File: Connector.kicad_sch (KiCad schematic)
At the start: 13 parts, among them J10 JST_XH_S2B-A, J3 JST_XH_S4B-A, J4 JST_XH_S2B-A, J5 JST_XH_S2B-A, J6 JST_XH_S2B-A, J7 JST_XH_S2B-A, J8 JST_XH_S3B, SW2 OS102011MA1Q, U13 74LVC2G126

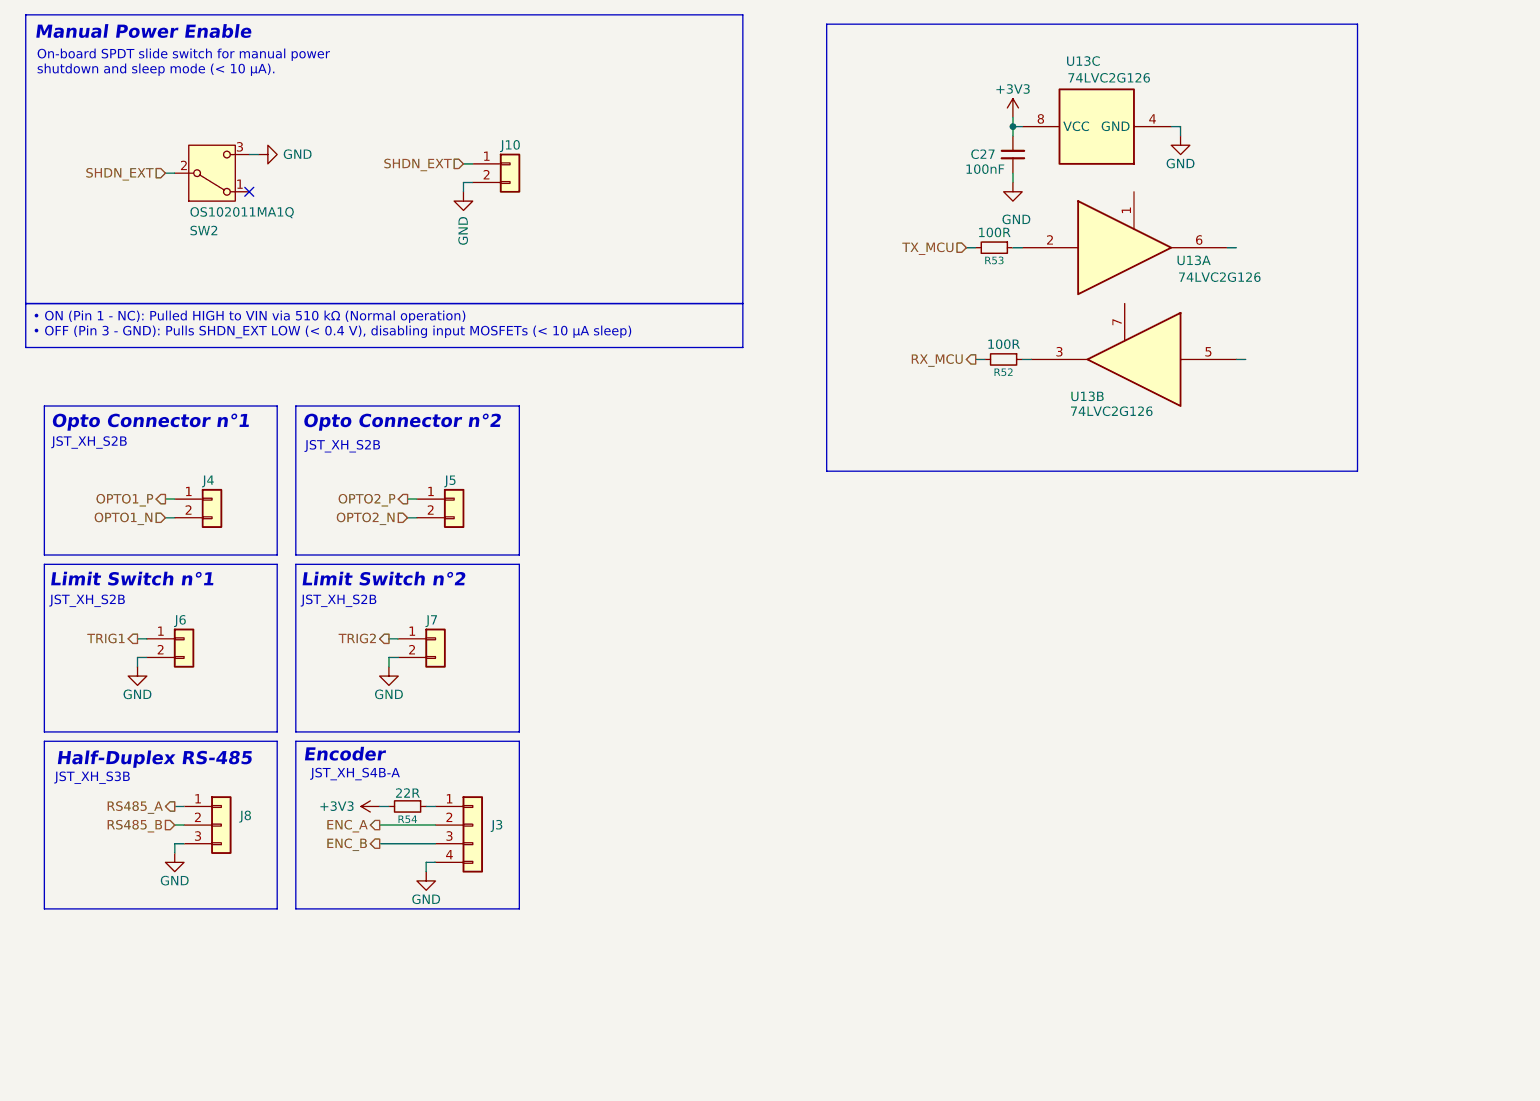
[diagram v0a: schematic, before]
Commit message: fix: FIx some modification
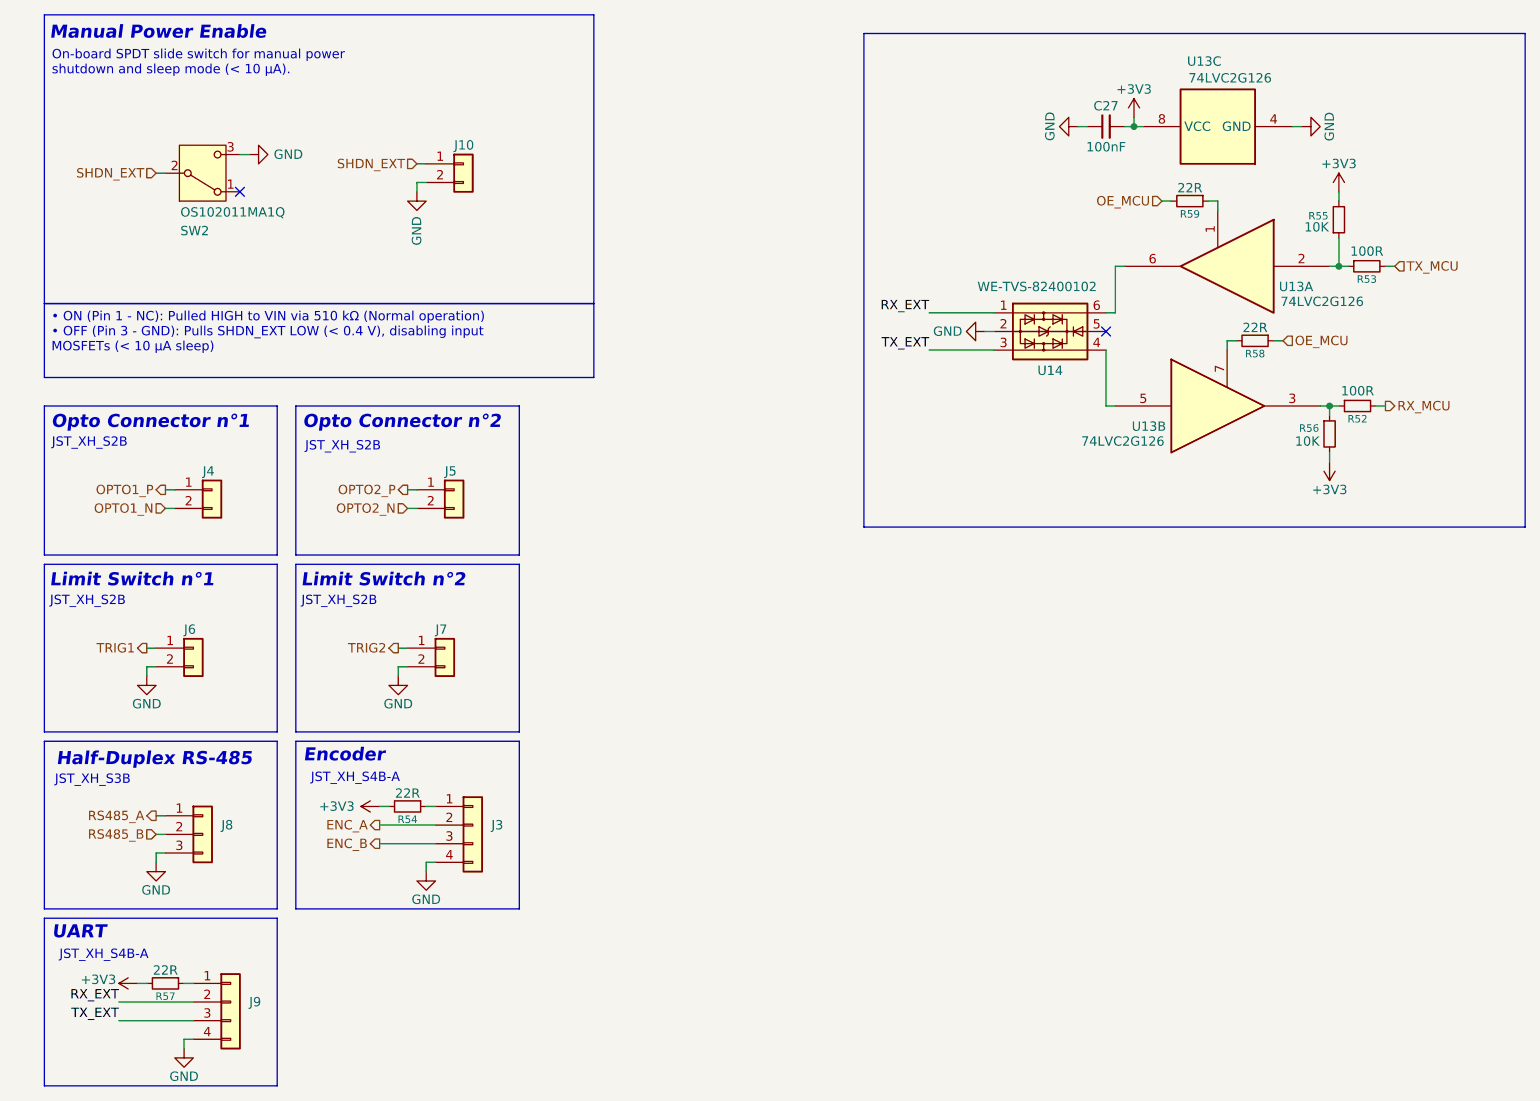
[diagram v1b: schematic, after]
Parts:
- added J9: JST_XH_S4B-A, Connector_JST:JST_XH_S4B-XH-A-1_1x04_P2.50mm_Horizontal, symbol Connector_Generic:Conn_01x04
- added R55, R56: 10K, Resistor_SMD:R_0603_1608Metric, symbol Device:R_Small
- added R57, R58, R59: 22R, Resistor_SMD:R_0603_1608Metric, symbol Device:R_Small
- added U14: WE-TVS-82400102, Package_TO_SOT_SMD:SOT-23-6, symbol Power_Protection:WE-TVS-82400102
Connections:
- net +3V3: now also R55.2, R56.2, R57.2
- net GND: now also J9.4 (Pin_4), U14.2
- net at R53.1, U13.2: now also R55.1
- net at U13.1: now also R59.1
- net at U13.6: now also U14.6
- net at R52.1, U13.3: now also R56.1
- net at U13.5: now also U14.4
- net at U13.7: now also R58.2
- new net: J9.1 (Pin_1), R57.1
- new net OE_MCU: R58.1, R59.2
- new net RX_EXT: J9.2 (Pin_2), U14.1
- new net TX_EXT: J9.3 (Pin_3), U14.3
- no-connect marks 1 -> 2
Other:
- note added: "UART"
- moved on the sheet: J10, J4, J5, J6, J7, J8, R52, R53, SW2, U13A, U13B, U13C
